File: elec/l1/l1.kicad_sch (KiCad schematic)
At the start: 107 parts, among them SW1 SW_Push, U1 CD74HC4067M, U10 XT30PW-F, U11 VNH5050A-E, U12 XT30PW-F, U2 CD74HC4067M, U4 STM32F103CBTx, U5 VNH5050A-E, U6 XT30PW-F, U7 VNH5050A-E, U8 XT30PW-F, U9 VNH5050A-E, Y1 8Mhz

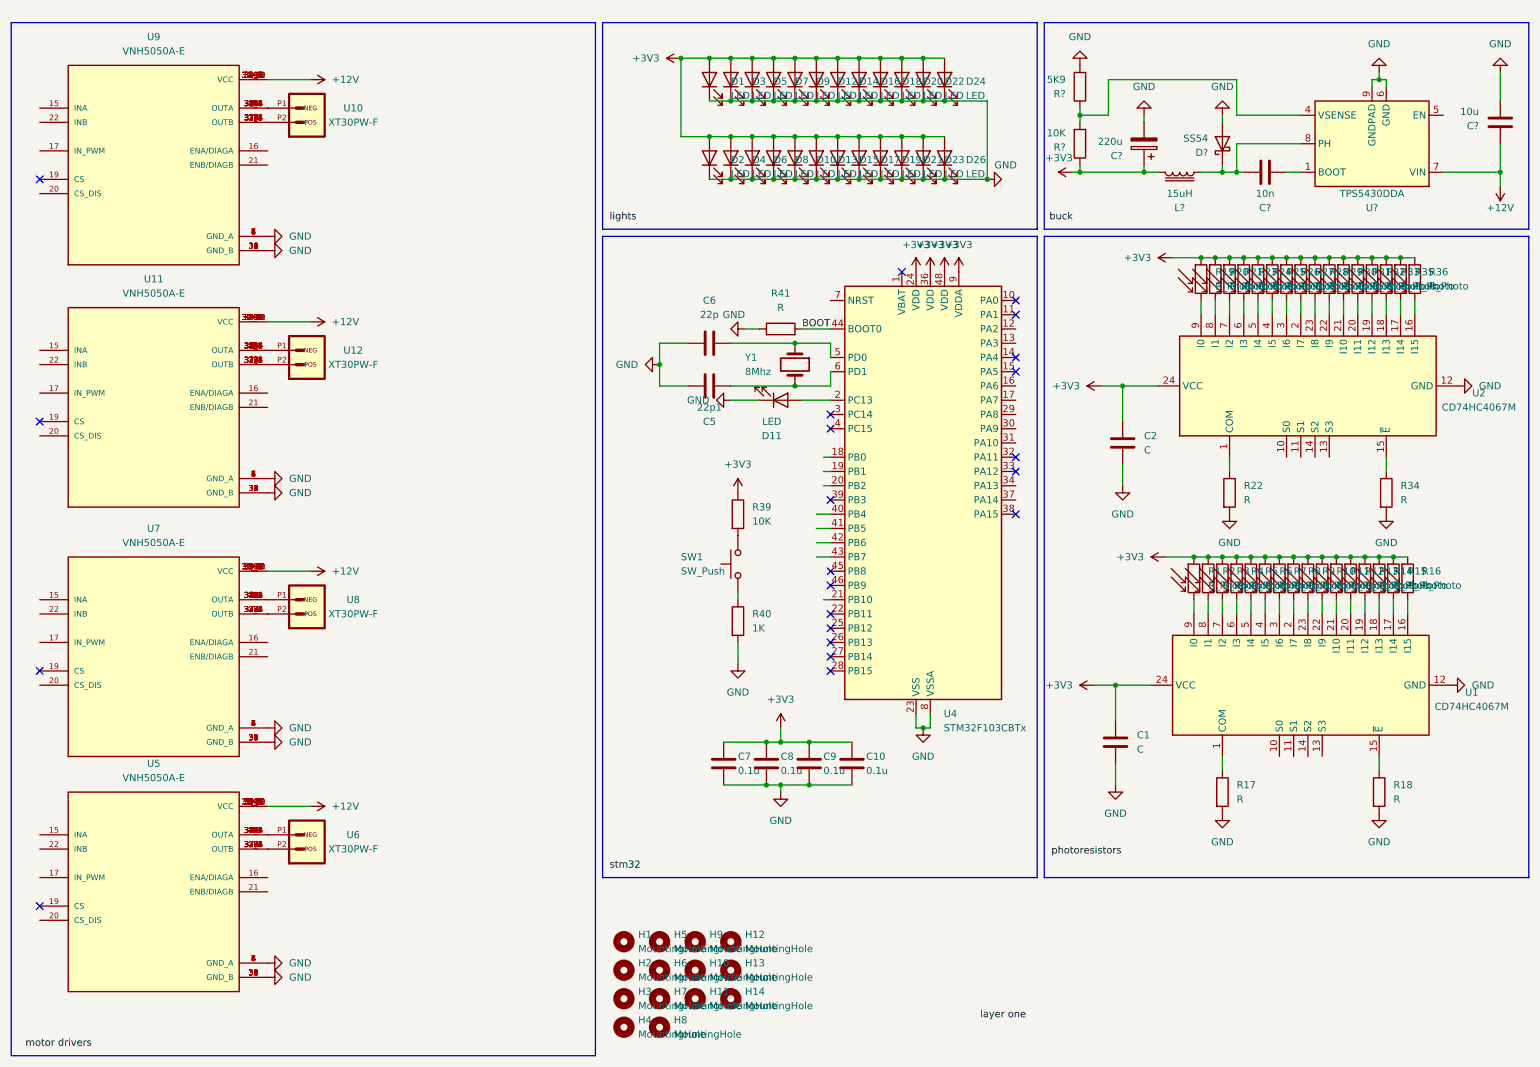
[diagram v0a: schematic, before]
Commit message: hamburger cheeseburger big mac whopper
hamburger cheeseburger
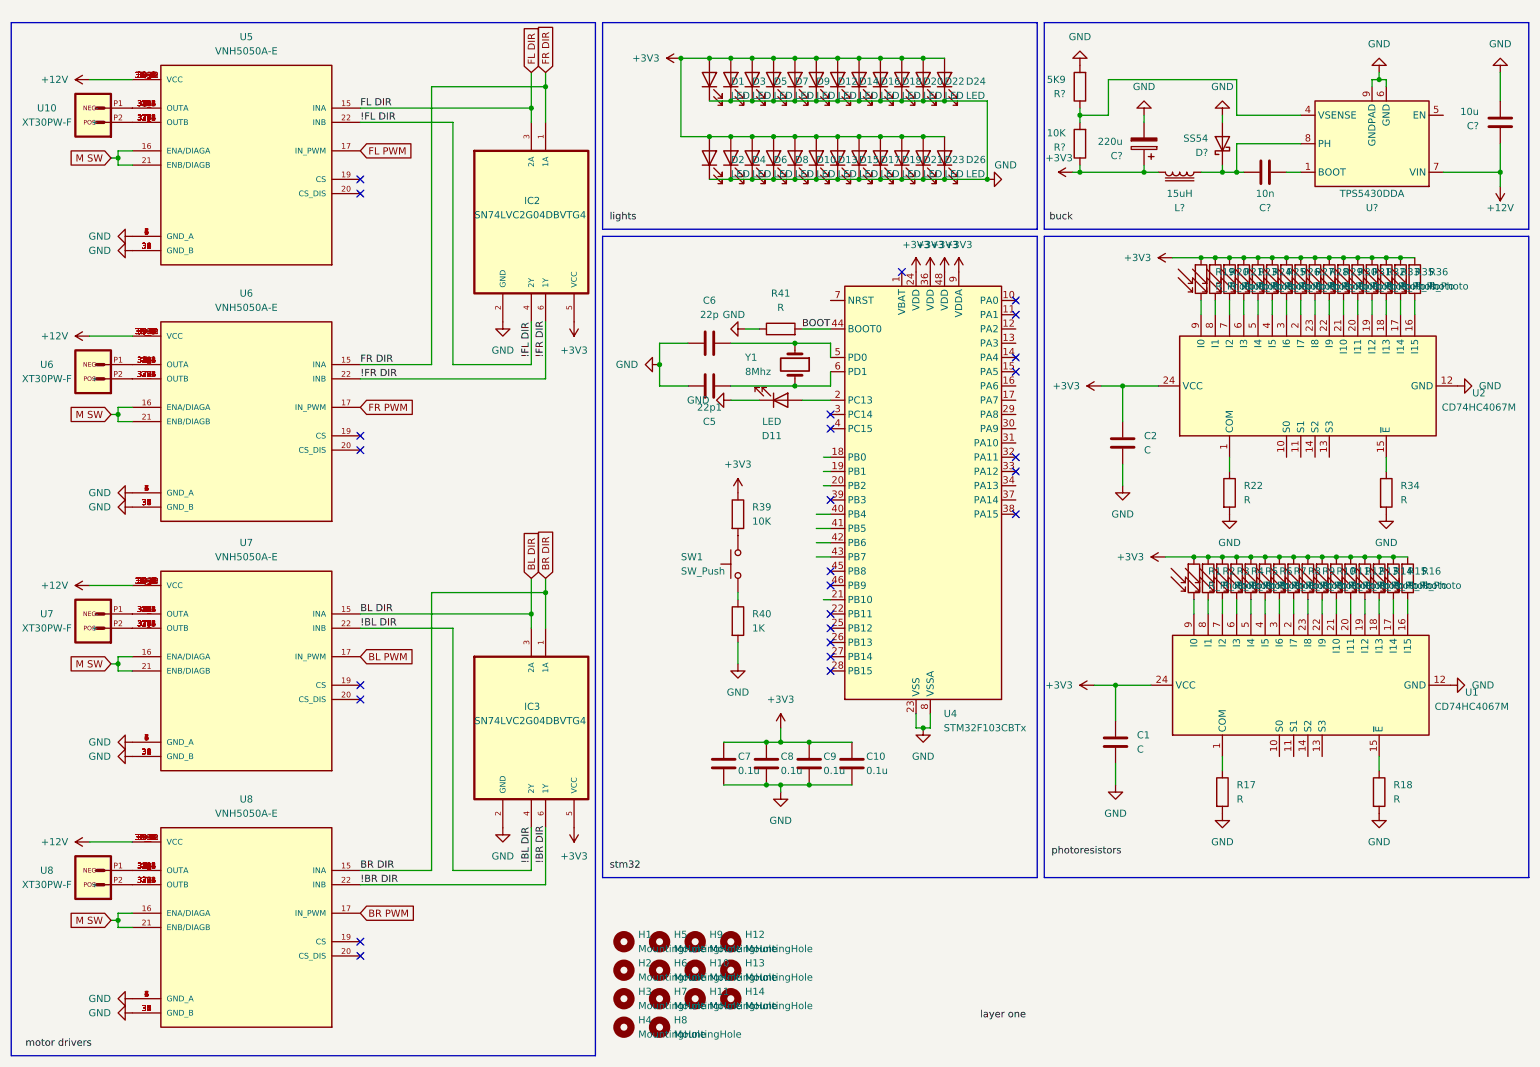
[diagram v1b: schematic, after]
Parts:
- removed U11, U5: VNH5050A-E, SOP50P1030X247-39N, symbol VNH5050A-E:VNH5050A-E
- removed U12: XT30PW-F, XT30PW-F, symbol XT30PW-F:XT30PW-F
- added IC2, IC3: SN74LVC2G04DBVTG4, SOT95P280X145-6N, symbol SN74LVC2G04DBVTG4:SN74LVC2G04DBVTG4
- added U6, U8: VNH5050A-E, SOP50P1030X247-39N, symbol VNH5050A-E:VNH5050A-E
- added U7: XT30PW-F, XT30PW-F, symbol XT30PW-F:XT30PW-F
- renumbered U9 to U5
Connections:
- net +12V: now also U6.13 (VCC), U6.24 (VCC), U6.39 (VCC), U6.39_1 (VCC), U6.39_10 (VCC), U6.39_11 (VCC), U6.39_12 (VCC), U6.39_2 (VCC), U6.39_3 (VCC), U6.39_4 (VCC), U6.39_5 (VCC), U6.39_6 (VCC), U6.39_7 (VCC), U6.39_8 (VCC), U6.39_9 (VCC), U8.13 (VCC), U8.24 (VCC), U8.39 (VCC), U8.39_1 (VCC), U8.39_10 (VCC), U8.39_11 (VCC), U8.39_12 (VCC), U8.39_2 (VCC), U8.39_3 (VCC), U8.39_4 (VCC), U8.39_5 (VCC), U8.39_6 (VCC), U8.39_7 (VCC), U8.39_8 (VCC), U8.39_9 (VCC)
- net +3V3: now also IC2.5 (VCC), IC3.5 (VCC)
- net GND: now also IC2.2 (GND), IC3.2 (GND), U6.1 (GND_A), U6.3 (GND_A), U6.30 (GND_B), U6.31 (GND_B), U6.32 (GND_B), U6.33 (GND_B), U6.34 (GND_B), U6.36 (GND_B), U6.4 (GND_A), U6.5 (GND_A), U6.6 (GND_A), U6.7 (GND_A), U8.1 (GND_A), U8.3 (GND_A), U8.30 (GND_B), U8.31 (GND_B), U8.32 (GND_B), U8.33 (GND_B), U8.34 (GND_B), U8.36 (GND_B), U8.4 (GND_A), U8.5 (GND_A), U8.6 (GND_A), U8.7 (GND_A)
- net at U7.10 (OUTA), U7.11 (OUTA), U7.12 (OUTA)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: now also U7.P1 (-); no longer U8.P1 (-)
- net BL DIR: now reaches U7.15 (INA)
- net BL DIR: now also IC3.3 (2A)
- net M SW: now reaches U7.16 (ENA/DIAGA)
- net M SW: now also U5.16 (ENA/DIAGA), U5.21 (ENB/DIAGB), U7.21 (ENB/DIAGB), U6.16 (ENA/DIAGA), U6.21 (ENB/DIAGB), U8.16 (ENA/DIAGA), U8.21 (ENB/DIAGB)
- net BL PWM: now reaches U7.17 (IN_PWM)
- net !BL DIR: now reaches U7.22 (INB)
- net !BL DIR: now also IC3.4 (2Y)
- net at U7.23 (OUTB), U7.25 (OUTB), U7.26 (OUTB)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: now also U7.P2 (+); no longer U8.P2 (+)
- net FL DIR: now reaches U5.15 (INA)
- net FL DIR: now also IC2.3 (2A)
- net FL PWM: now reaches U5.17 (IN_PWM)
- net !FL DIR: now reaches U5.22 (INB)
- net !FL DIR: now also IC2.4 (2Y)
- net at U6.P1 (-): now also U6.10 (OUTA), U6.11 (OUTA), U6.12 (OUTA), U6.14 (OUTA), U6.2 (OUTA), U6.38 (OUTA), U6.38_1 (OUTA), U6.38_2 (OUTA), U6.38_3 (OUTA), U6.38_4 (OUTA), U6.38_5 (OUTA), U6.38_6 (OUTA), U6.8 (OUTA), U6.9 (OUTA)
- net at U6.P2 (+): now also U6.23 (OUTB), U6.25 (OUTB), U6.26 (OUTB), U6.27 (OUTB), U6.28 (OUTB), U6.29 (OUTB), U6.35 (OUTB), U6.37 (OUTB), U6.37_1 (OUTB), U6.37_2 (OUTB), U6.37_3 (OUTB), U6.37_4 (OUTB), U6.37_5 (OUTB), U6.37_6 (OUTB)
- new net: U8.10 (OUTA), U8.11 (OUTA), U8.12 (OUTA), U8.14 (OUTA), U8.2 (OUTA), U8.38 (OUTA), U8.38_1 (OUTA), U8.38_2 (OUTA), U8.38_3 (OUTA), U8.38_4 (OUTA), U8.38_5 (OUTA), U8.38_6 (OUTA), U8.8 (OUTA), U8.9 (OUTA), U8.P1 (-)
- new net: U8.23 (OUTB), U8.25 (OUTB), U8.26 (OUTB), U8.27 (OUTB), U8.28 (OUTB), U8.29 (OUTB), U8.35 (OUTB), U8.37 (OUTB), U8.37_1 (OUTB), U8.37_2 (OUTB), U8.37_3 (OUTB), U8.37_4 (OUTB), U8.37_5 (OUTB), U8.37_6 (OUTB), U8.P2 (+)
- new net !BR DIR: IC3.6 (1Y), U8.22 (INB)
- new net !FR DIR: IC2.6 (1Y), U6.22 (INB)
- new net BR DIR: IC3.1 (1A), U8.15 (INA)
- new net BR PWM: U8.17 (IN_PWM)
- new net FR DIR: IC2.1 (1A), U6.15 (INA)
- new net FR PWM: U6.17 (IN_PWM)
- no-connect marks 22 -> 26
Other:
- moved on the sheet: U10, U5
